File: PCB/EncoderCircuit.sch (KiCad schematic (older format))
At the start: 10 parts, among them SW8 Rotary_Encoder_Switch

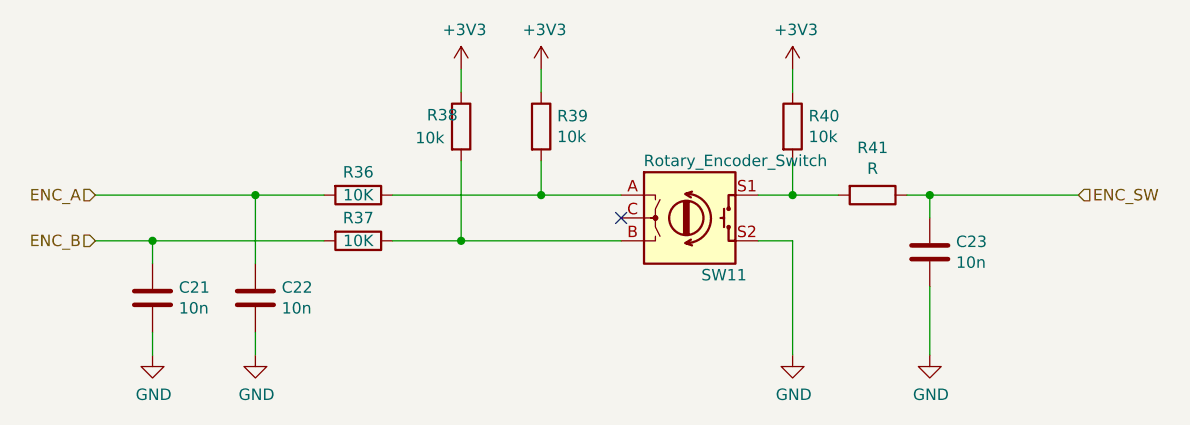
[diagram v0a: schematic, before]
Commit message: WIP PCB changes
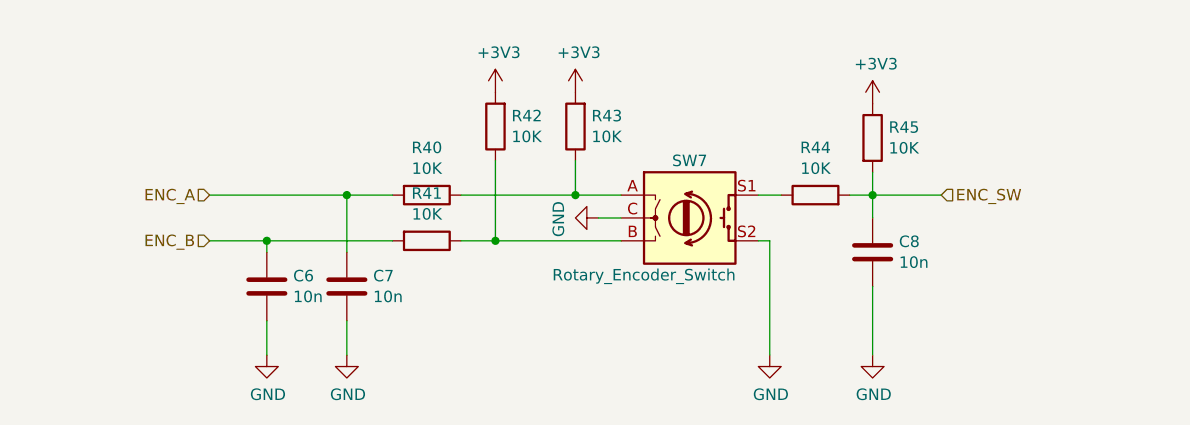
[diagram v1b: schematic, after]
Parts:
- removed R18, R19: 10K, symbol Device:R
- removed R20, R21, R22: 10k, symbol Device:R
- removed R23: R, symbol Device:R
- added R40, R41, R42, R43, R44, R45: 10K, Resistor_SMD:R_0402_1005Metric, symbol Device:R
- C6: renamed from C12; footprint (none) -> Capacitor_SMD:C_0402_1005Metric; Digikey (none) -> 311-1677-1-ND; MPN (none) -> CC0402JRX7R8BB103; Manufacturer (none) -> Yageo
- C7: renamed from C13; footprint (none) -> Capacitor_SMD:C_0402_1005Metric; Digikey (none) -> 311-1677-1-ND; MPN (none) -> CC0402JRX7R8BB103; Manufacturer (none) -> Yageo
- C8: renamed from C14; footprint (none) -> Capacitor_SMD:C_0402_1005Metric; Digikey (none) -> 311-1677-1-ND; MPN (none) -> CC0402JRX7R8BB103; Manufacturer (none) -> Yageo
- SW7: renamed from SW8; footprint (none) -> EMRSNxEOS:PEC12RHeader; Digikey (none) -> PEC11R-4220F-S0012-ND; MPN (none) -> PEC11R-4220F-S0012; Manufacturer (none) -> Bourns Inc.
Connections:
- net +3V3: now also R42.2, R43.2, R45.1
- net ENC_A: now also R40.2
- net ENC_B: now also R41.2
- net ENC_SW: now also R44.2, R45.2
- net GND: now also SW7.C
- net at SW7.A: now also R40.1, R43.1
- net at SW7.B: now also R41.1, R42.1
- net at SW7.S1: now also R44.1
- no-connect marks 1 -> 0
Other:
- moved on the sheet: C6, C7, C8
